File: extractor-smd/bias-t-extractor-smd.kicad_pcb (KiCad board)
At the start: 2 copper layers, 42 x 56 mm, 17 parts, among them J1 Conn_Coaxial, J2 Screw_Terminal_01x02, J3 Conn_Coaxial

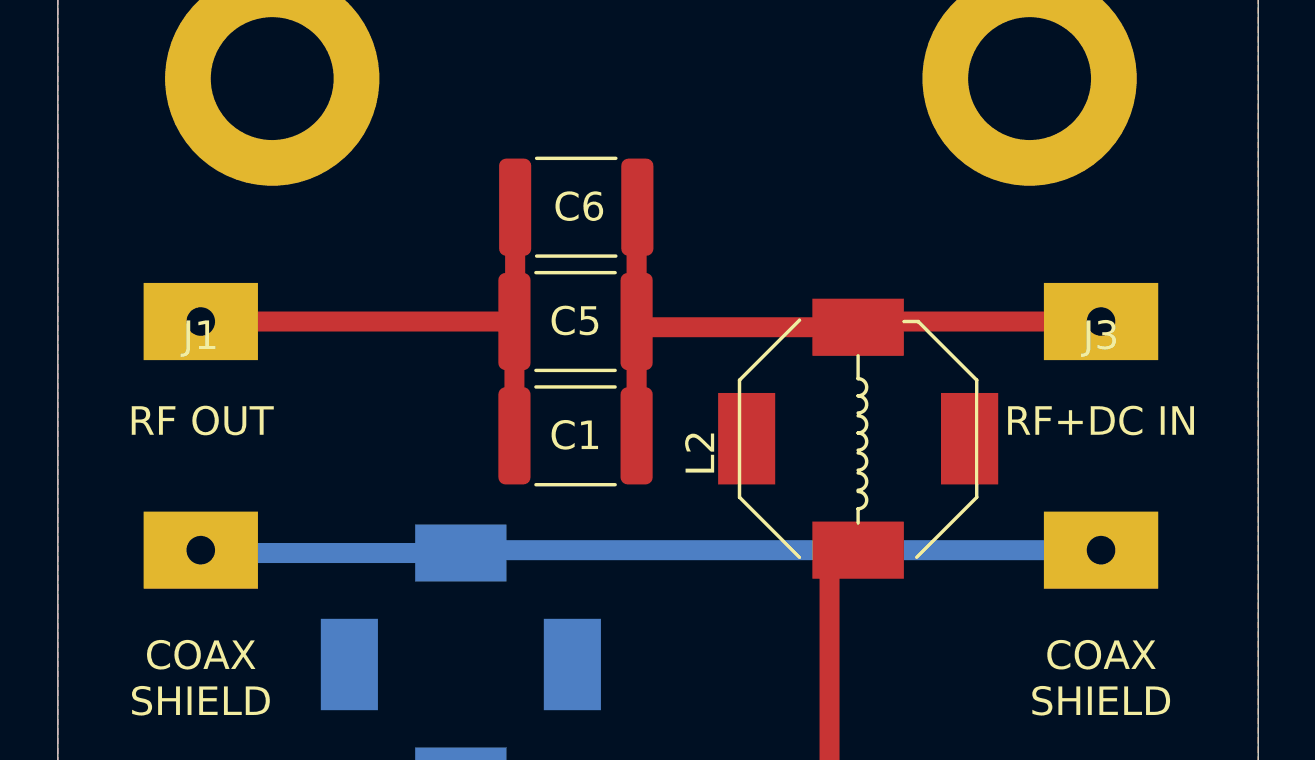
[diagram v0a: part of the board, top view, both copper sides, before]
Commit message: Add files via upload
Updated RF paths to 2.5mm with
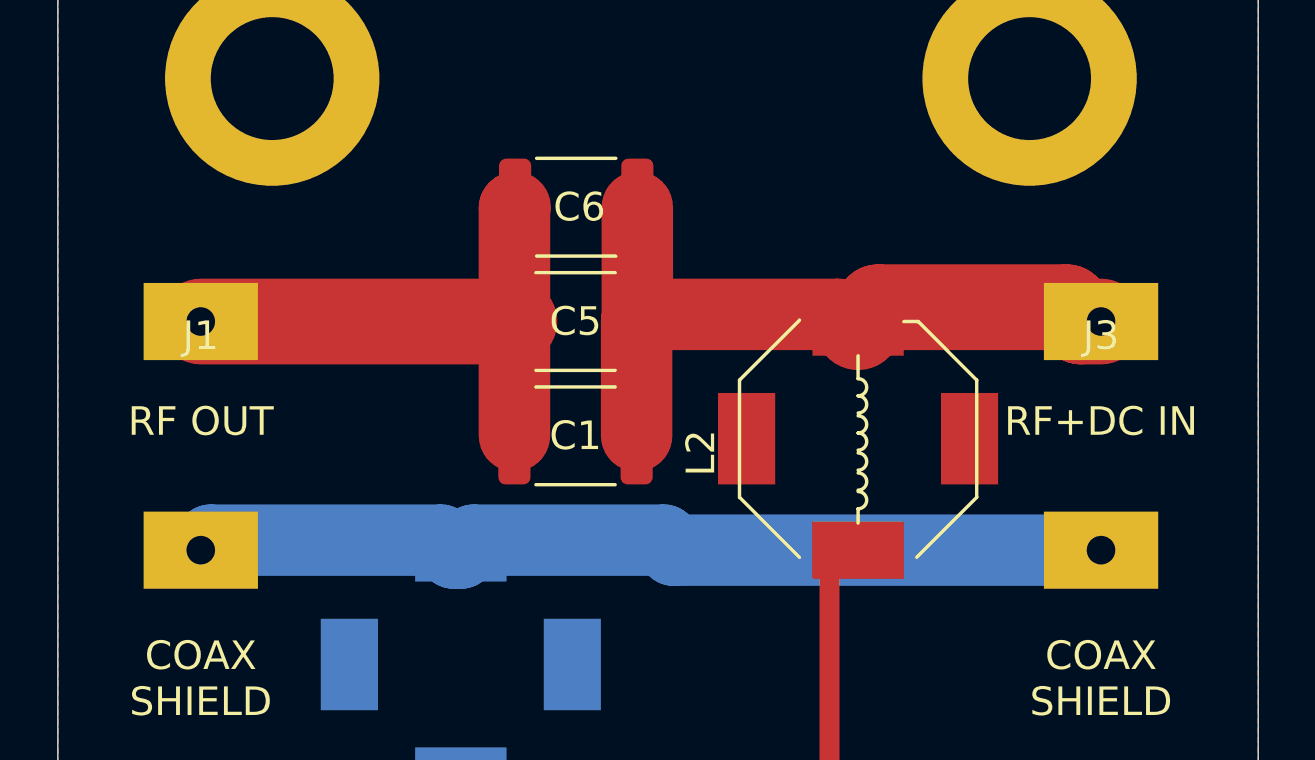
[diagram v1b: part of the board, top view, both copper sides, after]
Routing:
- net /RF+DC: track 24.4 -> 25.6 mm
- net /RF-GND: track 31.6 -> 32.4 mm
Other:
- net class RF: trace_width 0.7 -> 2.5
- net class RF-GND: trace_width 0.7 -> 2.5
